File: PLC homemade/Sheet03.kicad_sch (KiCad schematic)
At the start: 54 parts, among them IC4 MAX13487EESA+T, J1 M20-7820646, J16 Conn_01x04, J17 Conn_01x02, U11 GP8403-TC50-EW_C3152007, U4 LM324ADT, U5 SN74LVC1G125DRL, U6 SN74LVC1G125DRL

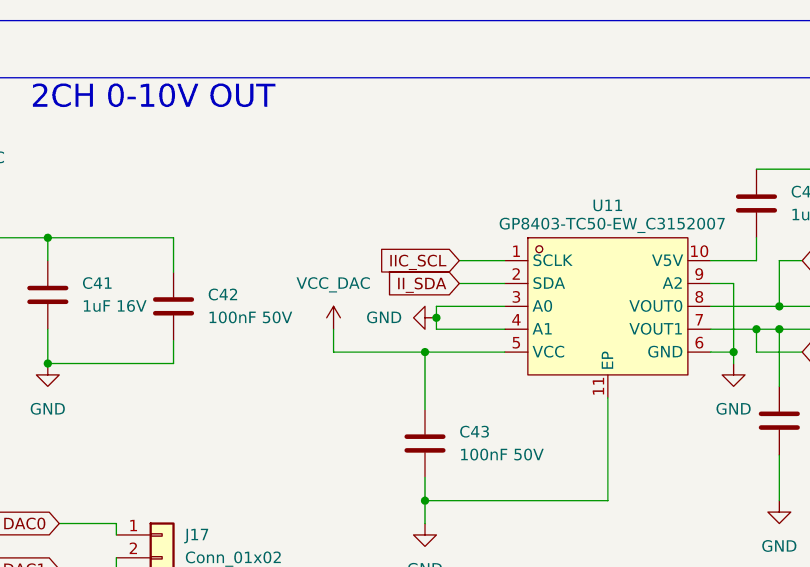
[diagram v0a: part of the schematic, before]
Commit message: :art: wiring componets done
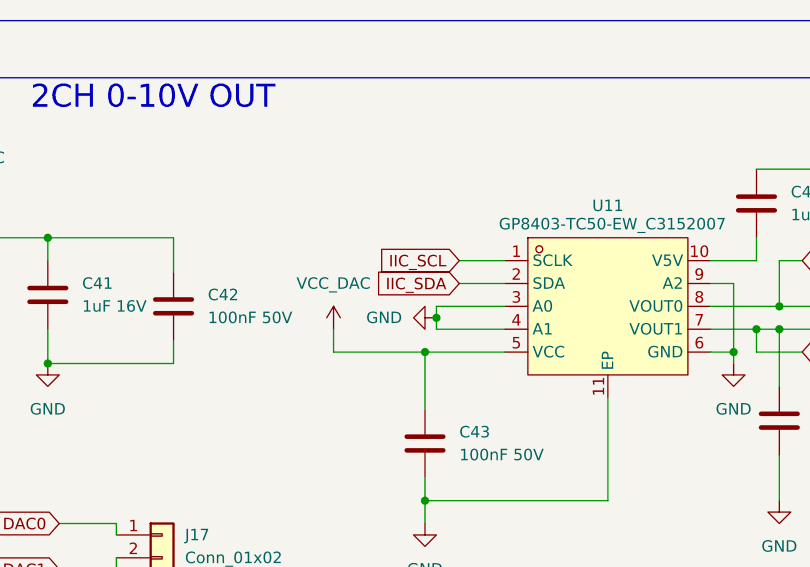
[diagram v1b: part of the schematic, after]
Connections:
- net II_SDA renamed IIC_SDA
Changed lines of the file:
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@@
-		)
-	)
-	(global_label "II_SDA"
-		(shape input)
-		(at 102.87 134.62 180)
-		(fields_autoplaced yes)
-		(effects
-			(font
-				(size 1.27 1.27)
-			)
-			(justify right)
-		)
-		(property "Intersheetrefs" "${INTERSHEET_REFS}"
-			(at 94.1395 134.62 0)
-			(effects
-				(font
-					(size 1.27 1.27)
-				)
-				(justify right)
-				(hide yes)
-			)
 		)
 	)
@@
 			(effects
 				(font
+					(size 1.27 1.27)
+				)
+				(justify right)
+				(hide yes)
+			)
+		)
+	)
+	(global_label "IIC_SDA"
+		(shape input)
+		(at 102.87 134.62 180)
+		(fields_autoplaced yes)
+		(effects
+			(font
+				(size 1.27 1.27)
+			)
+			(justify right)
+		)
+		(property "Intersheetrefs" "${INTERSHEET_REFS}"
+			(at 92.8695 134.62 0)
+			(effects
+				(font
